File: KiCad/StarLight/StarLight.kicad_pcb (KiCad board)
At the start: 2 copper layers, 81.3 x 103.1 mm, 77 parts, among them CN1 CN, Q1 Q_NPN, Q2 Q_NPN, Q3 Q_NPN, SW1 SW, SW2 SW

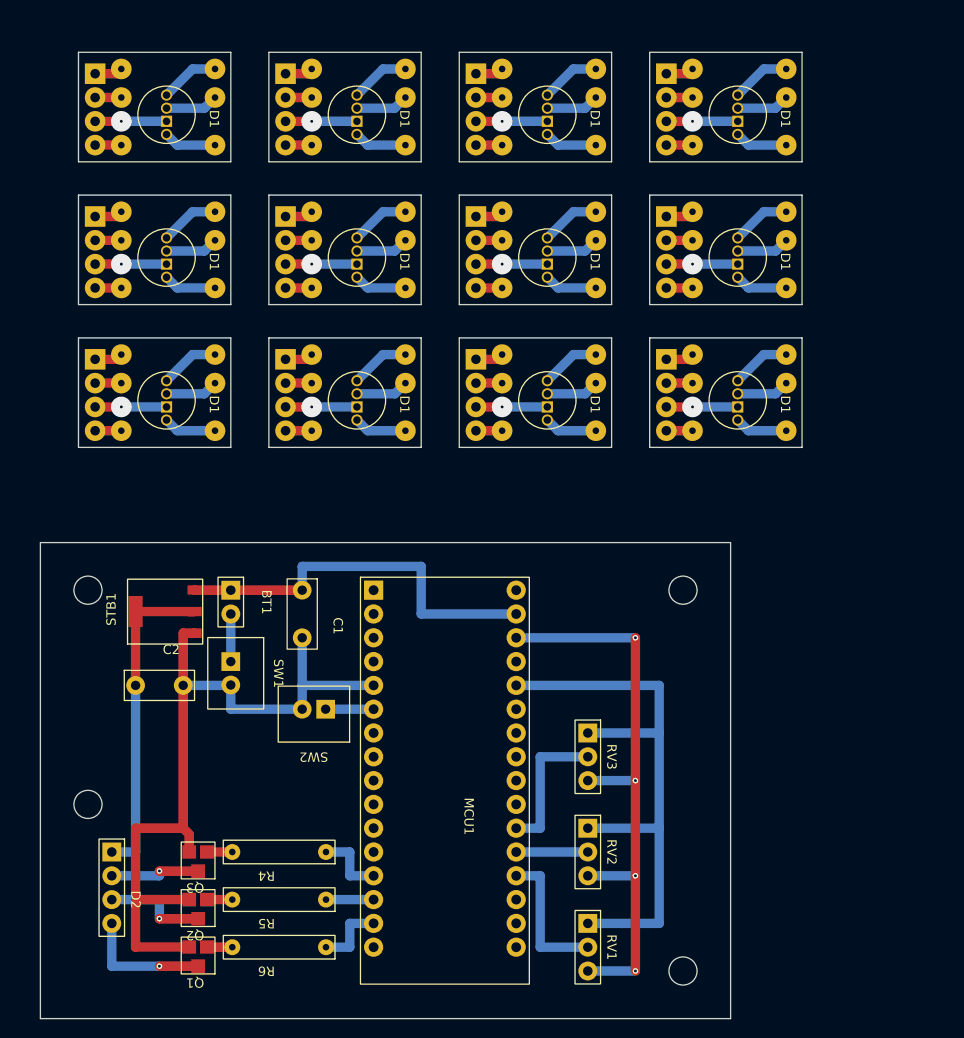
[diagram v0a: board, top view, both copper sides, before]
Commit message: replacement of seats
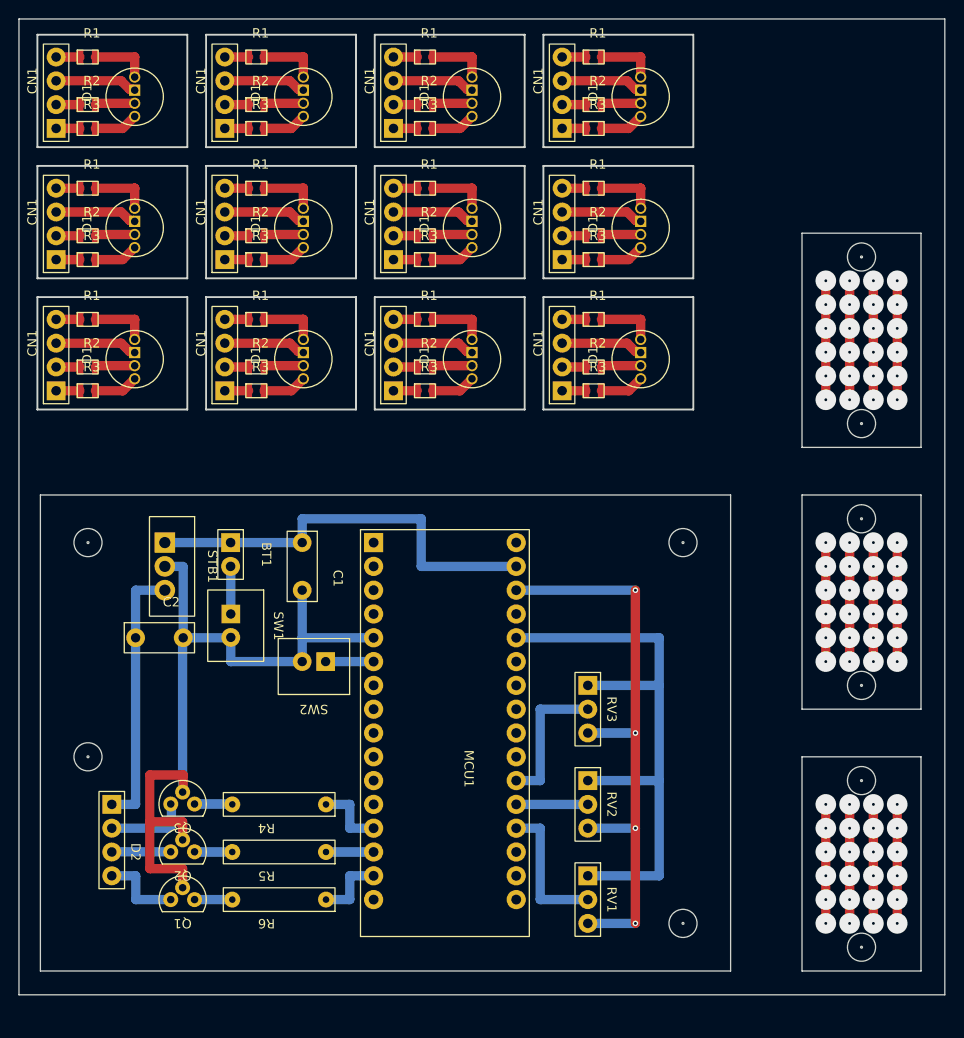
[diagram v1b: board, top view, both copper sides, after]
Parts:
- removed the CN1 at (46.5, 56.6)
- removed the CN1 at (26.2, 56.6)
- removed the CN1 at (66.8, 26.2)
- removed the CN1 at (66.8, 56.6)
- removed the CN1 at (87.1, 41.4)
- removed the CN1 at (87.1, 26.2)
- removed the CN1 at (46.5, 26.2)
- removed the CN1 at (46.5, 41.4)
- removed the CN1 at (66.8, 41.4)
- removed the CN1 at (26.2, 26.2)
- removed the CN1 at (26.2, 41.4)
- removed the CN1 at (87.1, 56.6)
- removed the D1 at (33.8, 58.9)
- removed the D1 at (54.1, 58.9)
- removed the D1 at (74.4, 43.7)
- removed the D1 at (54.1, 43.7)
- removed the D1 at (74.4, 58.9)
- removed the D1 at (33.8, 43.7)
- removed the D1 at (94.7, 43.7)
- removed the D1 at (94.7, 28.4)
- removed the D1 at (33.8, 28.4)
- removed the D1 at (54.1, 28.4)
- removed the D1 at (94.7, 58.9)
- removed the D1 at (74.4, 28.4)
- removed the R1 at (49.3, 64.3)
- removed the R1 at (89.9, 49.0)
- removed the R1 at (69.6, 64.3)
- removed the R1 at (89.9, 33.8)
- removed the R1 at (49.3, 33.8)
- removed the R1 at (69.6, 49.0)
- removed the R1 at (49.3, 49.0)
- removed the R1 at (69.6, 33.8)
- removed the R1 at (29.0, 49.0)
- removed the R1 at (29.0, 33.8)
- removed the R1 at (89.9, 64.3)
- removed the R1 at (29.0, 64.3)
- removed the R2 at (69.6, 28.7)
- removed the R2 at (29.0, 28.7)
- removed the R2 at (89.9, 43.9)
- removed the R2 at (89.9, 59.2)
- removed the R2 at (69.6, 43.9)
- removed the R2 at (49.3, 28.7)
- removed the R2 at (49.3, 59.2)
- removed the R2 at (29.0, 59.2)
- removed the R2 at (49.3, 43.9)
- removed the R2 at (69.6, 59.2)
- removed the R2 at (29.0, 43.9)
- removed the R2 at (89.9, 28.7)
- removed the R3 at (69.6, 40.9)
- removed the R3 at (49.3, 25.7)
- removed the R3 at (69.6, 25.7)
- removed the R3 at (29.0, 40.9)
- removed the R3 at (89.9, 56.1)
- removed the R3 at (69.6, 56.1)
- removed the R3 at (89.9, 25.7)
- removed the R3 at (49.3, 56.1)
- removed the R3 at (49.3, 40.9)
- removed the R3 at (29.0, 56.1)
- removed the R3 at (89.9, 40.9)
- removed the R3 at (29.0, 25.7)
- added CN1: CN, StarLightLayouts:PLS-4, F.Cu at (58.0, 60.0)
- added CN1: CN, StarLightLayouts:PLS-4, F.Cu at (58.0, 46.0)
- added CN1: CN, StarLightLayouts:PLS-4, F.Cu at (22.0, 46.0)
- added CN1: CN, StarLightLayouts:PLS-4, F.Cu at (76.0, 46.0)
- added CN1: CN, StarLightLayouts:PLS-4, F.Cu at (22.0, 60.0)
- added CN1: CN, StarLightLayouts:PLS-4, F.Cu at (76.0, 60.0)
- added CN1: CN, StarLightLayouts:PLS-4, F.Cu at (22.0, 32.0)
- added CN1: CN, StarLightLayouts:PLS-4, F.Cu at (58.0, 32.0)
- added CN1: CN, StarLightLayouts:PLS-4, F.Cu at (40.0, 46.0)
- added CN1: CN, StarLightLayouts:PLS-4, F.Cu at (40.0, 60.0)
- added CN1: CN, StarLightLayouts:PLS-4, F.Cu at (76.0, 32.0)
- added CN1: CN, StarLightLayouts:PLS-4, F.Cu at (40.0, 32.0)
- added D1: LED_ABGR, StarLightLayouts:RGB led, F.Cu at (84.4, 30.7)
- added D1: LED_ABGR, StarLightLayouts:RGB led, F.Cu at (48.4, 44.7)
- added D1: LED_ABGR, StarLightLayouts:RGB led, F.Cu at (66.4, 58.7)
- added D1: LED_ABGR, StarLightLayouts:RGB led, F.Cu at (48.4, 30.7)
- added D1: LED_ABGR, StarLightLayouts:RGB led, F.Cu at (30.4, 30.7)
- added D1: LED_ABGR, StarLightLayouts:RGB led, F.Cu at (30.4, 58.7)
- added D1: LED_ABGR, StarLightLayouts:RGB led, F.Cu at (84.4, 58.7)
- added D1: LED_ABGR, StarLightLayouts:RGB led, F.Cu at (84.4, 44.7)
- added D1: LED_ABGR, StarLightLayouts:RGB led, F.Cu at (30.4, 44.7)
- added D1: LED_ABGR, StarLightLayouts:RGB led, F.Cu at (66.4, 30.7)
- added D1: LED_ABGR, StarLightLayouts:RGB led, F.Cu at (48.4, 58.7)
- added D1: LED_ABGR, StarLightLayouts:RGB led, F.Cu at (66.4, 44.7)
- added R1: R, StarLightLayouts:SMD 0805, F.Cu at (78.5, 24.4)
- added R1: R, StarLightLayouts:SMD 0805, F.Cu at (60.5, 24.4)
- added R1: R, StarLightLayouts:SMD 0805, F.Cu at (42.5, 38.4)
- added R1: R, StarLightLayouts:SMD 0805, F.Cu at (24.5, 52.4)
- added R1: R, StarLightLayouts:SMD 0805, F.Cu at (42.5, 24.4)
- added R1: R, StarLightLayouts:SMD 0805, F.Cu at (42.5, 52.4)
- added R1: R, StarLightLayouts:SMD 0805, F.Cu at (78.5, 38.4)
- added R1: R, StarLightLayouts:SMD 0805, F.Cu at (60.5, 38.4)
- added R1: R, StarLightLayouts:SMD 0805, F.Cu at (78.5, 52.4)
- added R1: R, StarLightLayouts:SMD 0805, F.Cu at (60.5, 52.4)
- added R1: R, StarLightLayouts:SMD 0805, F.Cu at (24.5, 24.4)
- added R1: R, StarLightLayouts:SMD 0805, F.Cu at (24.5, 38.4)
- added R2: R, StarLightLayouts:SMD 0805, F.Cu at (42.5, 29.5)
- added R2: R, StarLightLayouts:SMD 0805, F.Cu at (60.5, 29.5)
- added R2: R, StarLightLayouts:SMD 0805, F.Cu at (42.5, 57.5)
- added R2: R, StarLightLayouts:SMD 0805, F.Cu at (78.5, 29.5)
- added R2: R, StarLightLayouts:SMD 0805, F.Cu at (60.5, 57.5)
- added R2: R, StarLightLayouts:SMD 0805, F.Cu at (78.5, 57.5)
- added R2: R, StarLightLayouts:SMD 0805, F.Cu at (24.5, 57.5)
- added R2: R, StarLightLayouts:SMD 0805, F.Cu at (24.5, 43.5)
- added R2: R, StarLightLayouts:SMD 0805, F.Cu at (42.5, 43.5)
- added R2: R, StarLightLayouts:SMD 0805, F.Cu at (24.5, 29.5)
- added R2: R, StarLightLayouts:SMD 0805, F.Cu at (60.5, 43.5)
- added R2: R, StarLightLayouts:SMD 0805, F.Cu at (78.5, 43.5)
- added R3: R, StarLightLayouts:SMD 0805, F.Cu at (78.5, 46.0)
- added R3: R, StarLightLayouts:SMD 0805, F.Cu at (78.5, 32.0)
- added R3: R, StarLightLayouts:SMD 0805, F.Cu at (42.5, 60.0)
- added R3: R, StarLightLayouts:SMD 0805, F.Cu at (60.5, 46.0)
- added R3: R, StarLightLayouts:SMD 0805, F.Cu at (24.5, 46.0)
- added R3: R, StarLightLayouts:SMD 0805, F.Cu at (60.5, 32.0)
- added R3: R, StarLightLayouts:SMD 0805, F.Cu at (42.5, 32.0)
- added R3: R, StarLightLayouts:SMD 0805, F.Cu at (78.5, 60.0)
- added R3: R, StarLightLayouts:SMD 0805, F.Cu at (42.5, 46.0)
- added R3: R, StarLightLayouts:SMD 0805, F.Cu at (24.5, 32.0)
- added R3: R, StarLightLayouts:SMD 0805, F.Cu at (24.5, 60.0)
- added R3: R, StarLightLayouts:SMD 0805, F.Cu at (60.5, 60.0)
- Q1, Q2, Q3: footprint StarLightLayouts:SOT23 -> StarLightLayouts:TO-92
- STB1: footprint StarLightLayouts:SOT-223 -> StarLightLayouts:TO-220
- moved STB1 10.2 mm to (33.6, 76.2), turned to -90 degrees
- moved Q3 5.29 mm to (36.8, 104.1)
- moved Q2 5.27 mm to (36.8, 109.2)
- moved Q1 5.23 mm to (36.8, 114.3)
- moved BT1 5.08 mm to (40.6, 76.2)
- moved RV2 5.08 mm to (78.7, 101.6)
- moved SW1 5.08 mm to (40.6, 83.8)
- moved C1 5.08 mm to (48.3, 76.2)
- moved C2 5.08 mm to (30.5, 86.4)
- moved D2 5.08 mm to (27.9, 104.1)
- moved MCU1 5.08 mm to (55.9, 76.2)
- moved R4 5.08 mm to (50.8, 104.1)
- moved R5 5.08 mm to (50.8, 109.2)
- moved R6 5.08 mm to (50.8, 114.3)
- moved RV1 5.08 mm to (78.7, 111.8)
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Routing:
- net (no net): track 0.00 -> 152.4 mm, vias 0 -> 72
- net Net-(D1-BK): track 75.9 -> 56.7 mm
- net Net-(D1-GK): track 67.8 -> 51.0 mm
- net Net-(D1-A): track 91.4 -> 105.6 mm, vias 12 -> 0
- net Net-(D1-RK): track 67.8 -> 76.0 mm
- net Net-(D2-A): track 34.5 -> 28.5 mm
- net Net-(CN1-PadBLUE): track 36.1 -> 30.5 mm
- net Net-(D2-RK): track 13.8 -> 8.81 mm, vias 1 -> 0
- net Net-(D2-GK): track 11.2 -> 6.30 mm, vias 1 -> 0
- net Net-(BT1-+): track 41.9 -> 45.1 mm
- net Net-(CN1-PadRED): track 33.5 -> 30.5 mm
- net Net-(CN1-PadGREEN): track 33.5 -> 30.5 mm
- net Net-(Q2-PadB): track 2.70 -> 4.57 mm
- net Net-(C1-Pad2): track 148.1 -> 146.4 mm
- net Net-(Q1-PadB): track 2.71 -> 4.03 mm
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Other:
- board size 81.3 x 103.1 mm -> 98.8 x 104.1 mm
